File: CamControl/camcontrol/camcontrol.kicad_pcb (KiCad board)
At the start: 4 copper layers, 27.9 x 27.9 mm, 75 parts, among them J2 USB_B_Micro, J3 Conn_01x03, J5 Conn_01x02, J6 Conn_01x02, J7 Conn_01x03, J8 Conn_01x04, Q2 AO3401A, Q3 AO3401A, U1 E22-900MM22S, U2 TPS1HC30BQPWPRQ1, U3 TPS63060DSCR, U4 XC6206P332MR, U5 W25Q128JVS, U6 RP2040, U7 TPS1HC30BQPWPRQ1, X1 SX1M12.000M10F30TNN

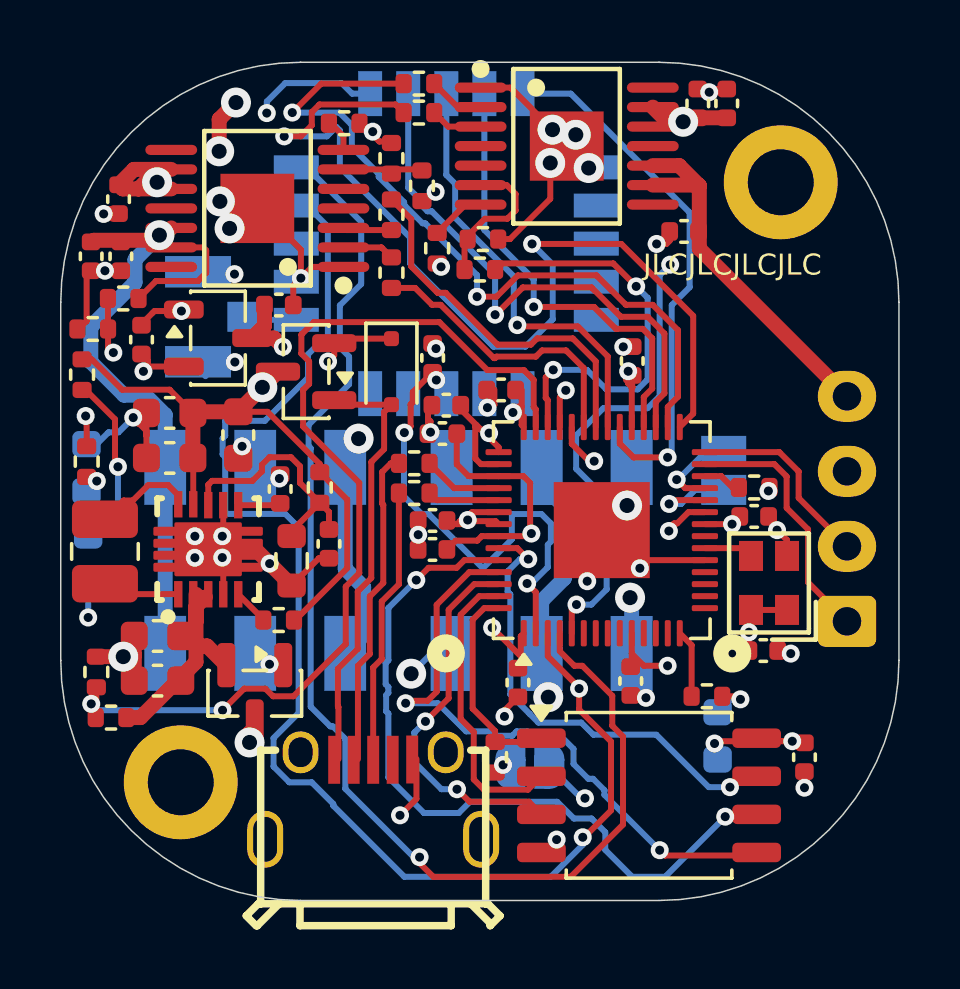
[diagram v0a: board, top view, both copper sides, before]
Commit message: cam control rework
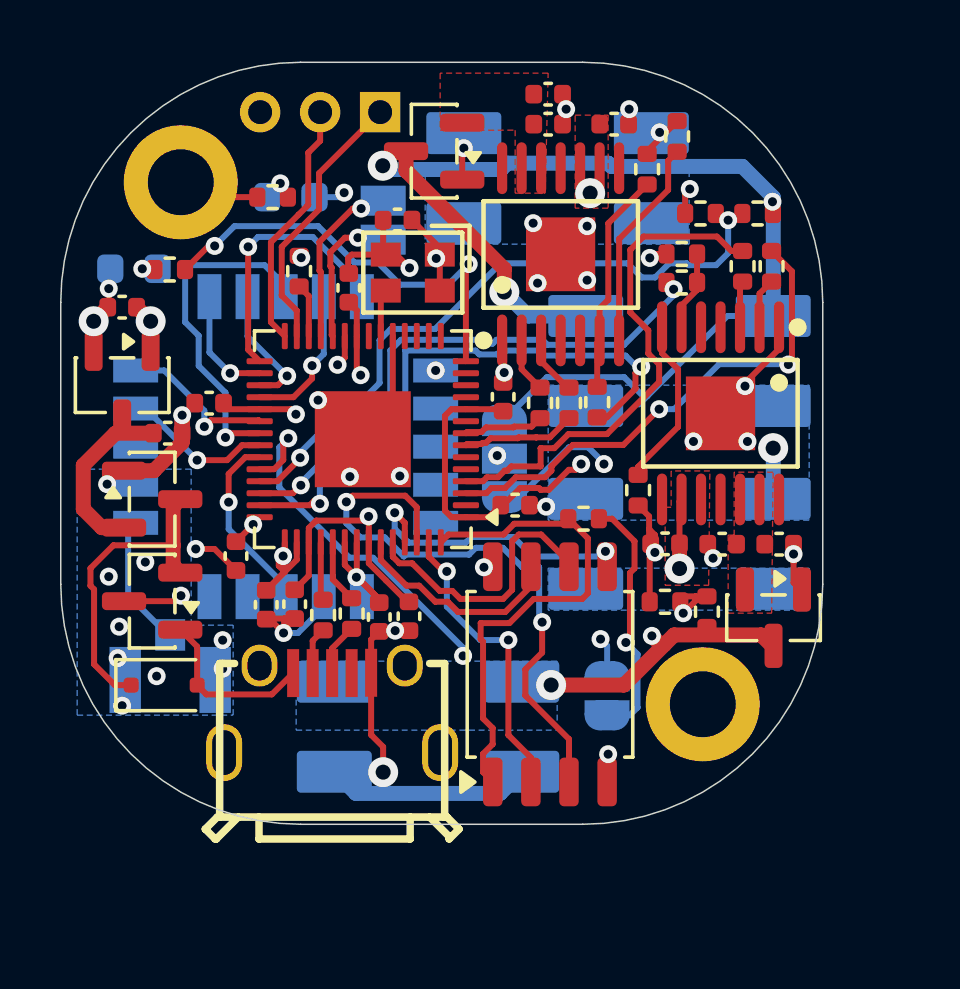
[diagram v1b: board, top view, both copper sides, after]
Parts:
- removed C1, C12, C7: 100n, Capacitor_SMD:C_0402_1005Metric
- removed C11, C9: 10u, Capacitor_SMD:C_0603_1608Metric
- removed C23, C24, C25: 22u, Capacitor_SMD:C_0603_1608Metric
- removed C8: 10p, Capacitor_SMD:C_0402_1005Metric
- removed D2: LED, LED_SMD:LED_0603_1608Metric
- removed L1: 1uH, Inductor_SMD:L_1008_2520Metric
- removed R10: 111k, Resistor_SMD:R_0603_1608Metric
- removed R13, R2: 1M, Resistor_SMD:R_0402_1005Metric
- removed R22: 1k, Resistor_SMD:R_0402_1005Metric
- removed U3: TPS63060DSCR, .pretty:WSON-10_L3.0-W3.0-P0.50-BL-EP-A
- added J1: Power 1, .pretty:wago2pin3mmspace, B.Cu at (174.3, 144.7)
- added J4: Power 1, .pretty:wago2pin3mmspace, B.Cu at (182.7, 132.5)
- added JP1: Jumper, Jumper:SolderJumper-3_P1.3mm_Open_RoundedPad1.0x1.5mm, B.Cu at (173.7, 133.1)
- added Q1: AO3401A, Package_TO_SOT_SMD:SOT-23, F.Cu at (162.0, 134.4)
- added Q4: AO3401A, Package_TO_SOT_SMD:SOT-23, F.Cu at (171.4, 122.8)
- J3, J7: value Conn_01x03 -> Power 1; footprint footprints:CONN3_2059-303&slash_998-403_WAG -> .pretty:wago2pin3mmspace
- J8: value Conn_01x04 -> Conn_01x03; footprint Connector_JST:JST_EH_B4B-EH-A_1x04_P2.50mm_Vertical -> Connector_PinHeader_2.00mm:PinHeader_1x03_P2.00mm_Vertical
- moved R7 27.3 mm to (182.2, 124.9)
- moved R8 25.3 mm to (180.3, 124.9), turned to 180 degrees
- moved D3 24.9 mm to (161.4, 126.7), turned to 180 degrees
- moved C28 23.9 mm to (182.9, 135.9), turned to 0 degrees
- moved C29 23.1 mm to (181.0, 135.9), turned to 180 degrees
- moved J8 23.0 mm to (169.6, 121.5)
- moved R9 22.9 mm to (162.6, 126.7), turned to 180 degrees
- moved R23 22.1 mm to (180.5, 138.2), turned to 90 degrees
- moved C30 21.5 mm to (179.1, 135.9), turned to 180 degrees
- moved R24 21.1 mm to (179.1, 137.8)
- moved H1 20.0 mm to (163.0, 123.8)
- moved C14 18.8 mm to (170.2, 125.1), turned to 180 degrees
- moved H2 17.6 mm to (180.4, 141.2)
- moved Q2 17.5 mm to (182.7, 138.4)
- moved J3 17.4 mm to (182.7, 138.6)
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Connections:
- C26 pad 1: +5V -> /12VIN
- C28 pad 1: +12V -> /12VAIN
- C29 pad 1: +12V -> /12VAIN
- C4 pad 1: +5V -> /12VIN
- C5 pad 1: Net-(D4-K) -> Net-(Q1-S)
- D1 pad 1: GND -> Net-(D1-K)
- D1 pad 2: Net-(D1-A) -> +3V3
- J3 pad 2: /VIDPWR -> GND
- J7 pad 1: GND -> /CAMPWR
- Q2 pad 2: /BATT POSTSW -> /12VAIN
- Q2 pad 3: +BATT -> +12V
- Q3 pad 3: +5V -> Net-(JP1-C)
- R1 pad 1: Net-(D1-A) -> Net-(D1-K)
- R1 pad 2: +3V3 -> GND
- R7 pad 1: /BATT POSTSW -> +12VA
- U2 pad 12: +5V -> /12VIN
- U2 pad 13: +5V -> /12VIN
- U4 pad 3: Net-(D4-K) -> Net-(Q1-S)
- U6 pad 2: /SX RST -> unconnected-(U6-GPIO0-Pad2)
- U6 pad 29: /CAM DIAG EN -> /SCLK
- U6 pad 3: /TXEN -> /VID EN
- U6 pad 30: /CAM EN -> /BUSY
- U6 pad 34: /SCLK -> /RXEN
- U6 pad 36: /VID DIAG EN -> /TXEN
- U6 pad 37: /VID EN -> /SX RST
- U6 pad 39: /VIDSNS -> /CAM BATT SENSE 
- U6 pad 4: /RXEN -> /VID DIAG EN
- U6 pad 40: /CAMSNS -> /VIDSNS
- U6 pad 41: /CAM BATT SENSE  -> /CAMSNS
- U6 pad 5: /BUSY -> unconnected-(U6-GPIO3-Pad5)
- U6 pad 7: unconnected-(U6-GPIO5-Pad7) -> /CAM DIAG EN
- U6 pad 8: unconnected-(U6-GPIO6-Pad8) -> /CAM EN
- U7 pad 12: +12V -> /12VAIN
- U7 pad 13: +12V -> /12VAIN
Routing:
- net +5V: track 49.4 -> 0.00 mm, vias 4 -> 0
- net /TXEN: track 45.0 -> 5.05 mm, vias 2 -> 1
- net +12VA: track 0.00 -> 38.4 mm, vias 0 -> 3
- net /RXEN: track 42.1 -> 5.32 mm
- net /BUSY: track 40.5 -> 3.82 mm, vias 3 -> 1
- net /CAM DIAG EN: track 31.6 -> 3.81 mm, vias 2 -> 0
- net /VIDPWR: track 25.7 -> 2.32 mm, vias 2 -> 1
- net /CAM EN: track 24.9 -> 2.68 mm, vias 2 -> 0
- net +BATT: track 21.7 -> 0.00 mm, vias 2 -> 0
- net /QSPI_SCLK: track 24.2 -> 9.30 mm, vias 2 -> 0
- net Net-(JP1-C): track 0.00 -> 14.9 mm, vias 0 -> 2
- net /MISO: track 18.5 -> 4.23 mm
- net /CAMPWR: track 12.4 -> 0.00 mm, vias 0 -> 1
- net /LEDINDICATION: track 2.26 -> 14.4 mm, vias 0 -> 2
- net /QSPI_SDO: track 20.9 -> 9.30 mm
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- added copper zone on B.Cu, net +12V
- added copper zone on F.Cu, net /12VAIN
- added copper zone on F.Cu, net /12VIN
- added copper zone on B.Cu, net /CAMPWR
- added copper zone on F.Cu, net /CAMPWR
- added copper zone on B.Cu, net /VIDPWR
- added copper zone on F.Cu, net /VIDPWR
- added copper zone on B.Cu, net GND
- added copper zone on In2.Cu, net GND
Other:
- board size 27.9 x 27.9 mm -> 25.4 x 25.4 mm
